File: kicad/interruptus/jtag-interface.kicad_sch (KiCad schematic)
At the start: 15 parts, among them J3 USB4110GFA, U4 FT2232D, Y1 6 MHz

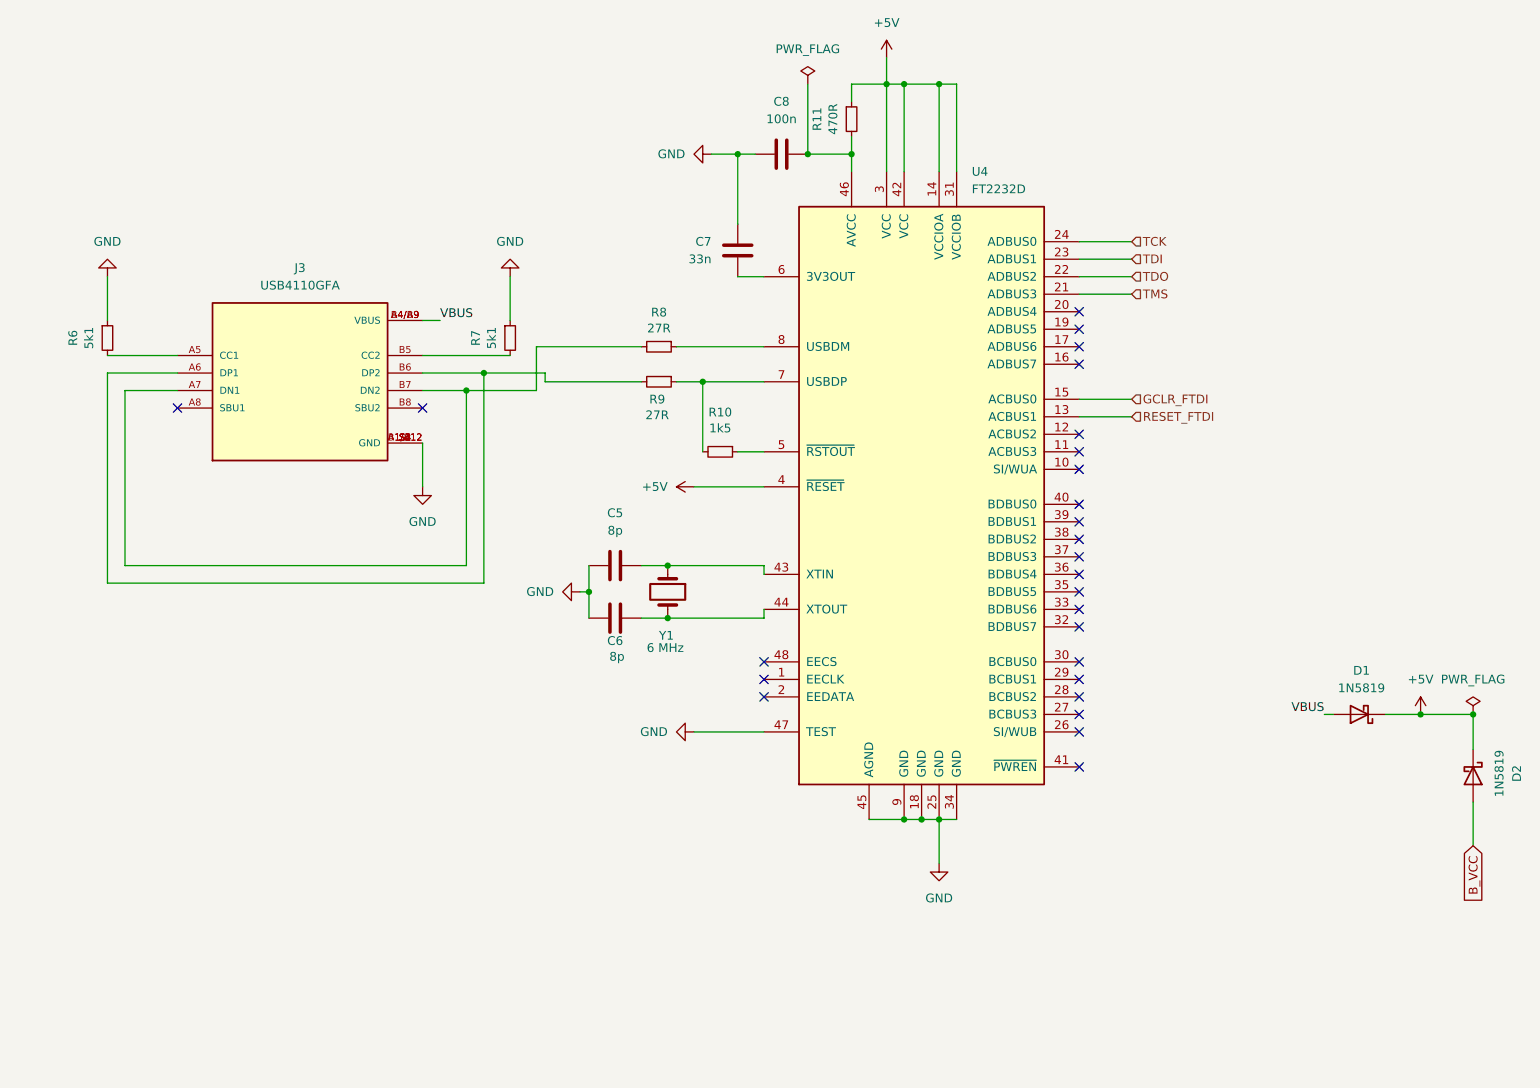
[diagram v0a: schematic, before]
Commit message: rev 5
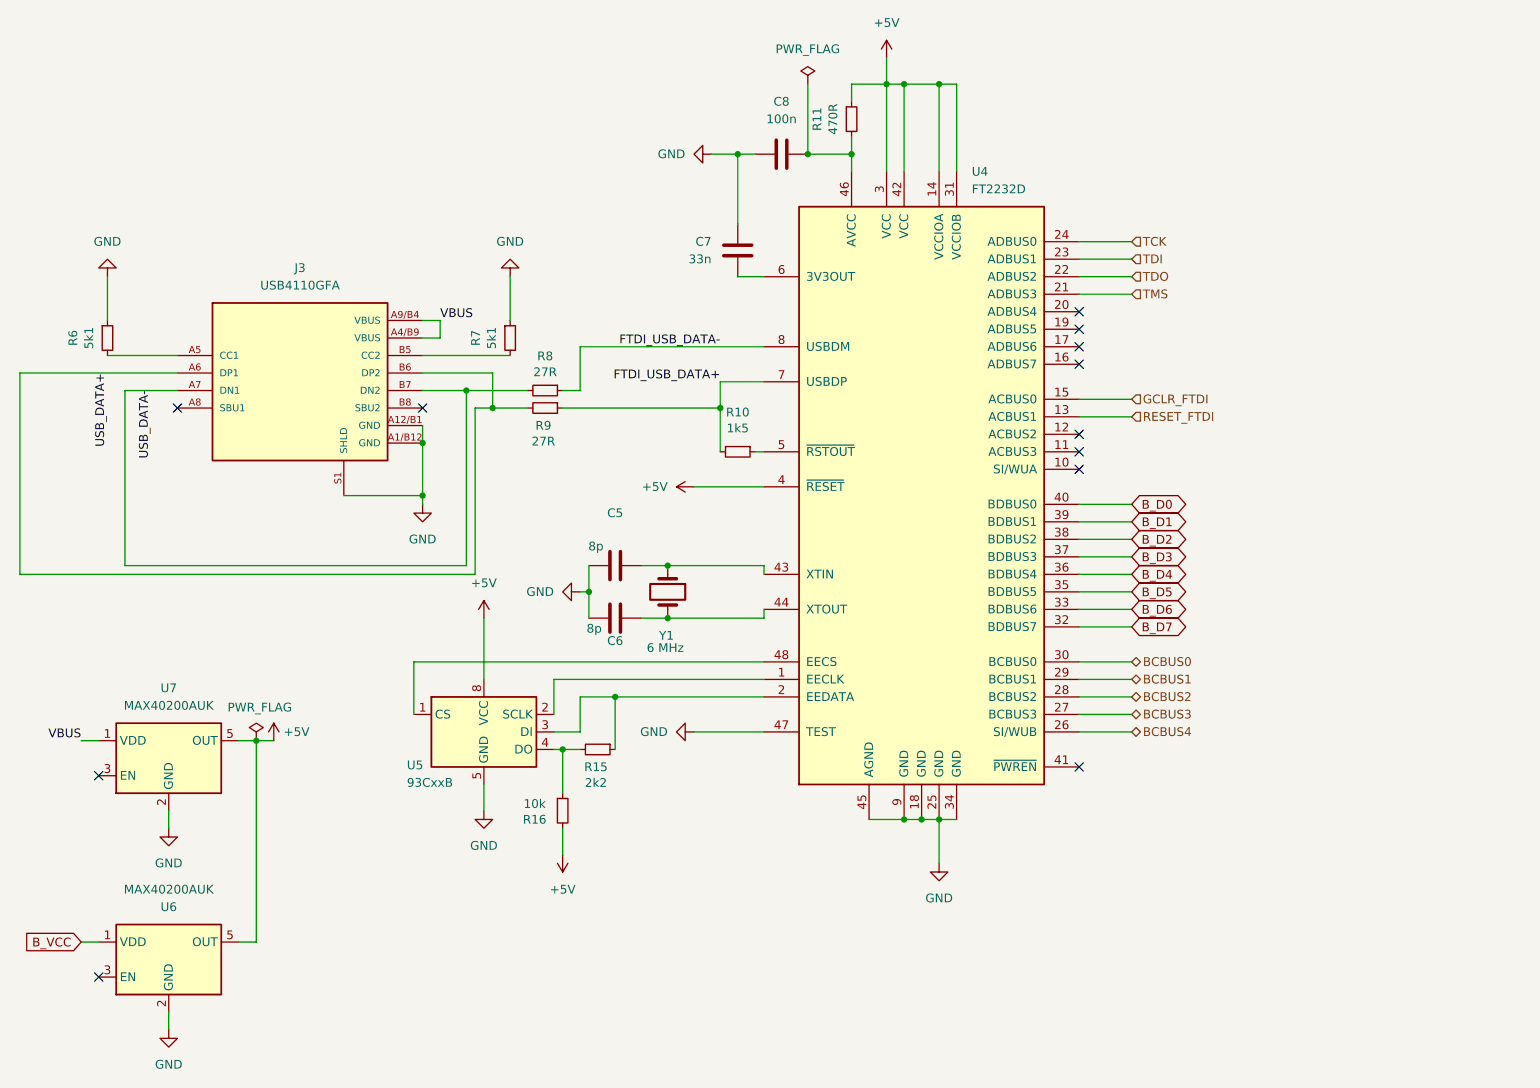
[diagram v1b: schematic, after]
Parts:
- removed D1, D2: 1N5819, Diode_SMD:Nexperia_CFP3_SOD-123W, symbol Diode:1N5819
- added R15: 2k2, Resistor_SMD:R_0201_0603Metric_Pad0.64x0.40mm_HandSolder, symbol Device:R_Small
- added R16: 10k, Resistor_SMD:R_0201_0603Metric_Pad0.64x0.40mm_HandSolder, symbol Device:R_Small
- added U5: 93CxxB, Package_SO:SOIC-8_3.9x4.9mm_P1.27mm, symbol Memory_EEPROM:93CxxB
- added U6, U7: MAX40200AUK, Package_TO_SOT_SMD:SOT-23-5, symbol Analog_Switch:MAX40200AUK
- J3: footprint Connector_USB:USB_C_Receptacle_GCT_USB4110 -> Library:USB_C_Receptacle_GCT_USB4110
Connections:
- net +5V: now also R16.2, U5.8 (VCC), U6.5 (OUT), U7.5 (OUT)
- net B_VCC: now also U6.1 (VDD)
- net GND: now also J3.A12/B1 (GND), U5.5 (GND), U6.2 (GND), U7.2 (GND); no longer J3.B1/A12 (GND), J3.S2 (GND), J3.S3 (GND), J3.S4 (GND)
- net VBUS: now also J3.A9/B4 (VBUS), U7.1 (VDD); no longer J3.B4/A9 (VBUS)
- net FTDI_USB_DATA-: now reaches R8.1, U4.8 (USBDM)
- net USB_DATA-: now reaches J3.A7 (DN1), J3.B7 (DN2), R8.2
- net USB_DATA+: now reaches J3.A6 (DP1), J3.B6 (DP2), R9.2
- net at U4.1 (EECLK): now also U5.2 (SCLK)
- net at U4.2 (EEDATA): now also R15.1, U5.3 (DI)
- net BCBUS4: now reaches U4.26 (SI/WUB)
- net BCBUS3: now reaches U4.27 (BCBUS3)
- net BCBUS2: now reaches U4.28 (BCBUS2)
- net BCBUS1: now reaches U4.29 (BCBUS1)
- net BCBUS0: now reaches U4.30 (BCBUS0)
- net B_D7: now reaches U4.32 (BDBUS7)
- net B_D6: now reaches U4.33 (BDBUS6)
- net B_D5: now reaches U4.35 (BDBUS5)
- net B_D4: now reaches U4.36 (BDBUS4)
- net B_D3: now reaches U4.37 (BDBUS3)
- net B_D2: now reaches U4.38 (BDBUS2)
- net B_D1: now reaches U4.39 (BDBUS1)
- net B_D0: now reaches U4.40 (BDBUS0)
- net at U4.48 (EECS): now also U5.1 (CS)
- net FTDI_USB_DATA+: now reaches R10.2, R9.1, U4.7 (USBDP)
- new net: R15.2, R16.1, U5.4 (DO)
- no-connect marks 26 -> 12
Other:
- moved on the sheet: R10, R8, R9
